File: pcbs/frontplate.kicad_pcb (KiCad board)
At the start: 2 copper layers, 133.3 x 91.7 mm, 5 parts

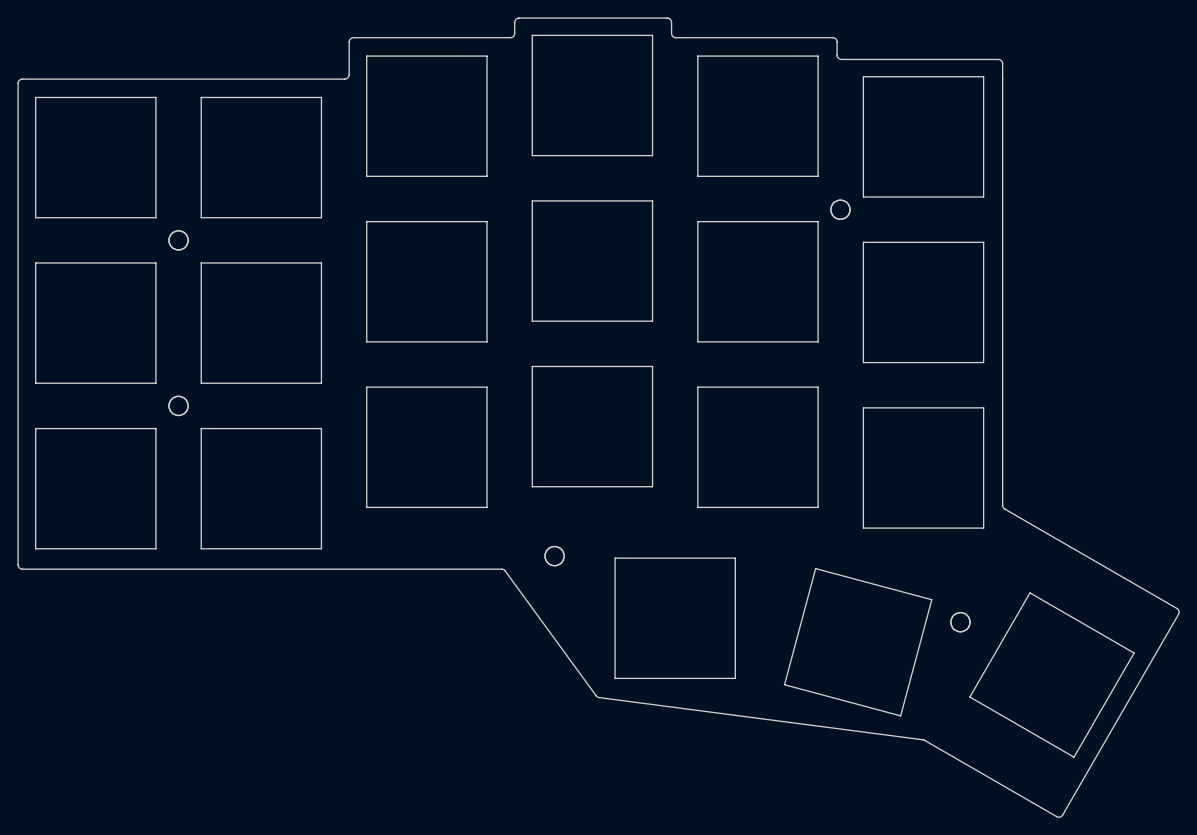
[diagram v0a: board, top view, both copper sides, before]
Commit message: build: regenerate outlines and PCBs with Ergogen snapshot
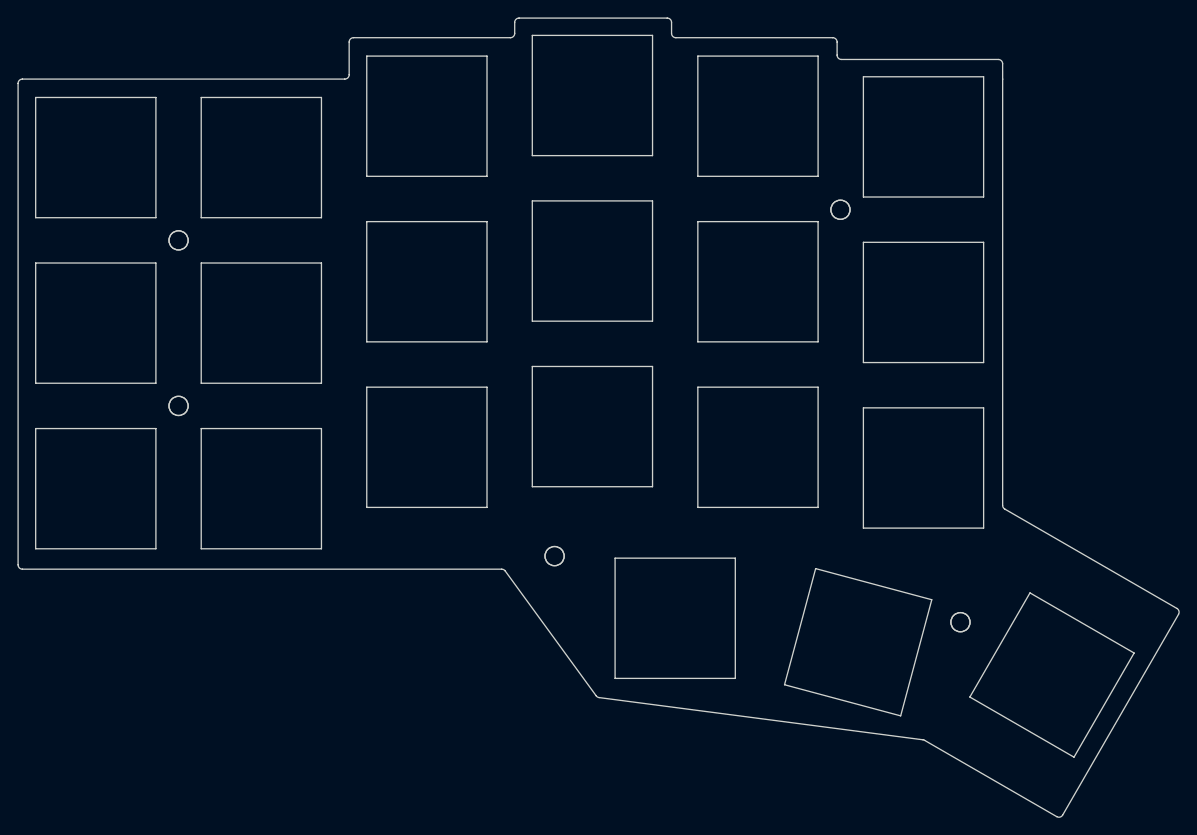
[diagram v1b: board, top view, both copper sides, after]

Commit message: build: regenerate PCBs, images, and gerbers
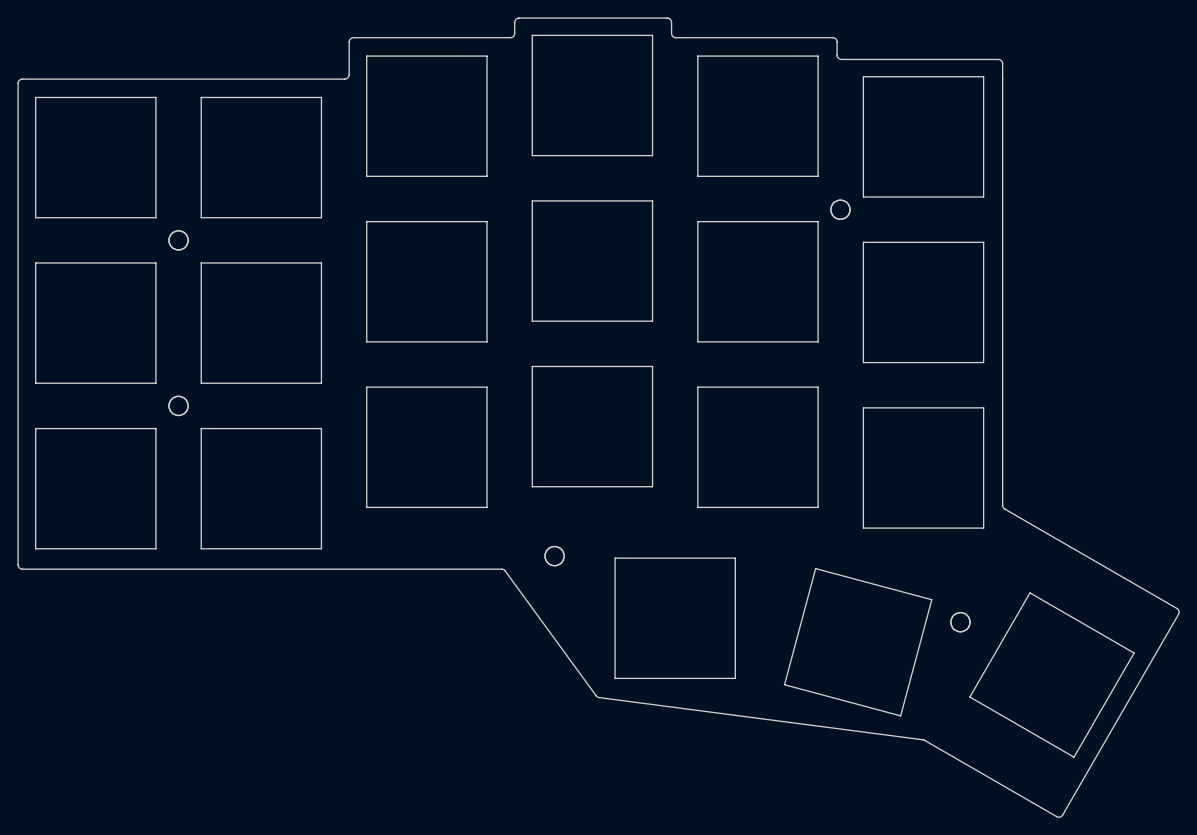
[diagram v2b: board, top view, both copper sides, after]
